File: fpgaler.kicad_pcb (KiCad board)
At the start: 4 copper layers, 100 x 100 mm, 287 parts, among them J1 USB_C_Receptacle_USB2.0, J3 JTAG, J4 FTDI_RST, J5 VGA, J6 DB9 Expander, J7 DB9 Expander, Q1 BC817, SW1 RotaryEncoder_Switch, SW2 RotaryEncoder_Switch, SW3 K1, SW4 K2, SW5 PROGRAMN, SW6 K3, SW7 FPGA GSRN, SW8 K4, U1 TLV62569DRL, U10 XC6206PxxxMR, U11 IS62WV51216BLL-55TLI, U2 TLV62569DRL, U3 NCP115-2.5, U5 93LC56BT-I/OT, U6 FT2232HL, U7 CAT24C128, U8 LFE5U-25F-8MG285C, U9 W25Q128JVP, X1 27MHz, Y1 7M-12.000MAAJ

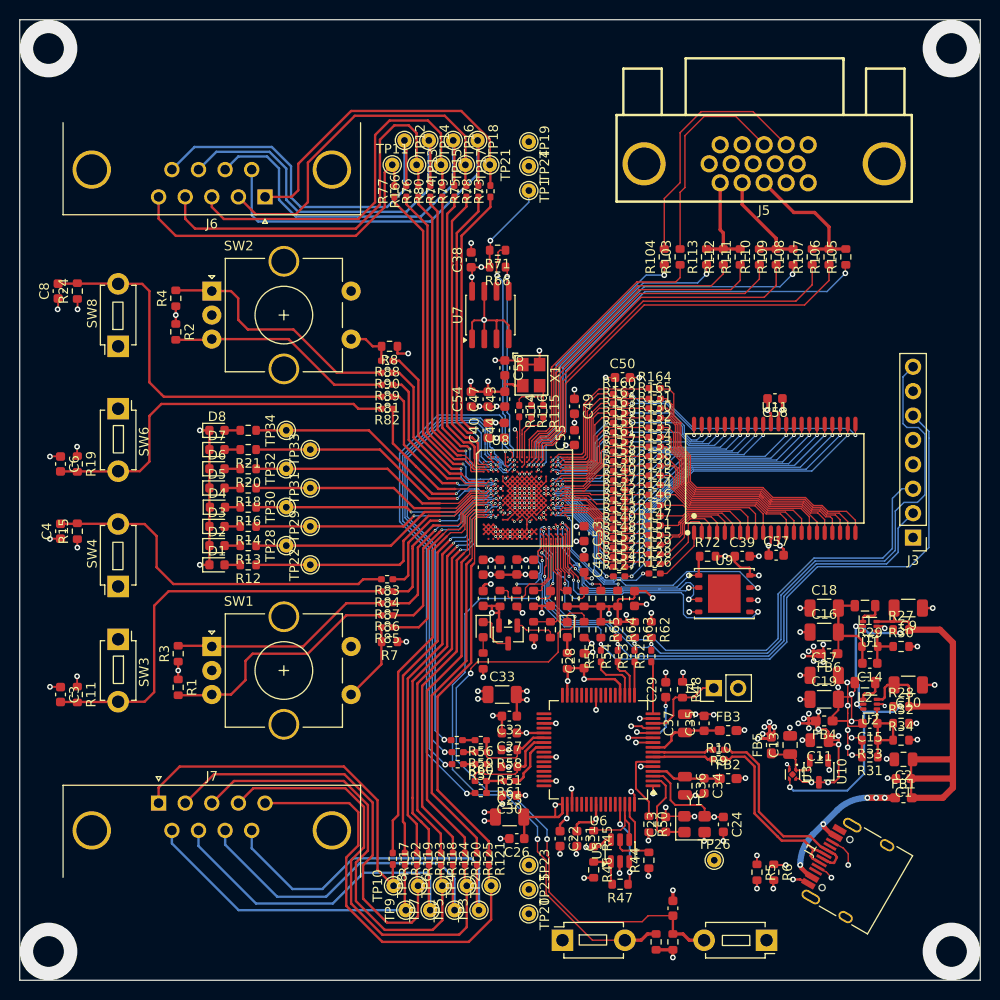
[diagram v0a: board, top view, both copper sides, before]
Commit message: Place planes
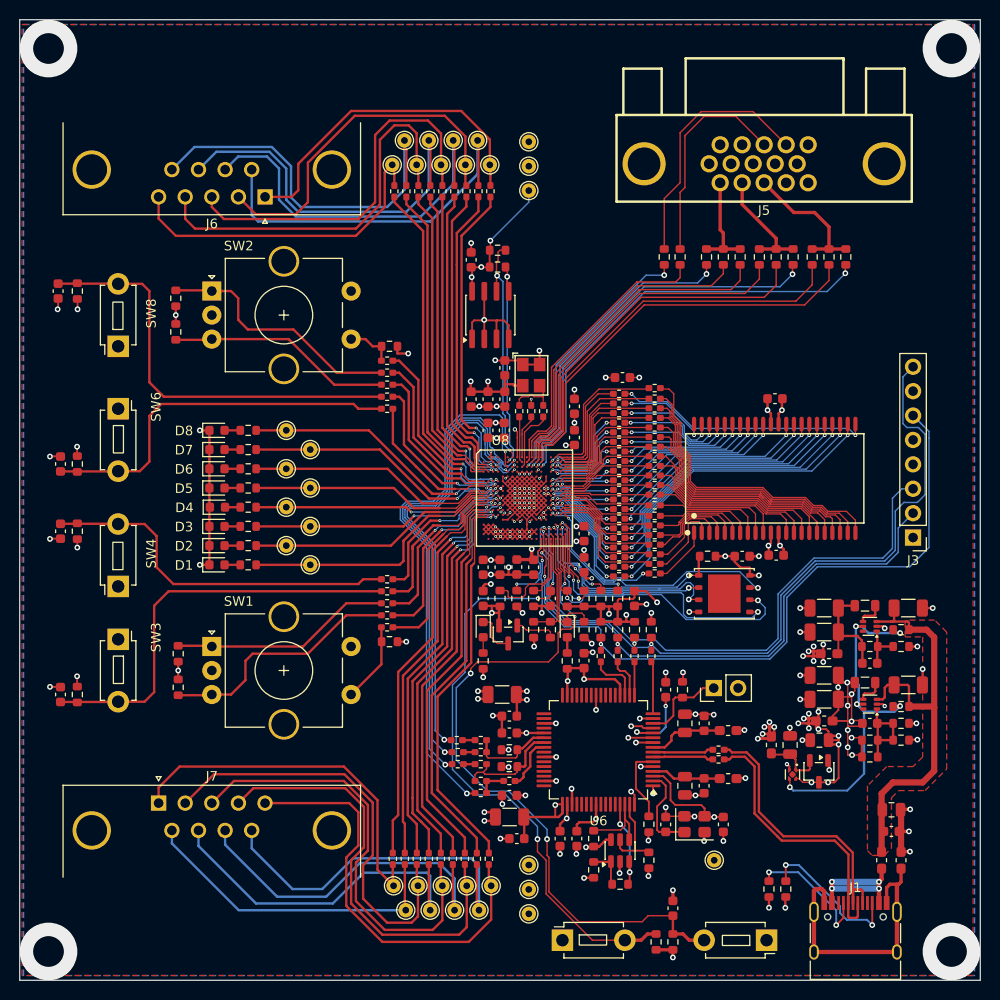
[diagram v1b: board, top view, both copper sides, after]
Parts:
- added FB7: 15Ω@100MHz, Inductor_SMD:L_0603_1608Metric_Pad1.05x0.95mm_HandSolder, F.Cu at (171.8, 132.5)
- moved FB1 6.89 mm to (169.7, 132.5), turned to 90 degrees
- moved J1 6.85 mm to (167.0, 141.0), turned to 0 degrees
- moved C1 5.64 mm to (170.8, 129.5), turned to 0 degrees
- moved C2 5.40 mm to (170.8, 127.2), turned to 0 degrees
- moved R5 3.47 mm to (159.8, 135.5)
- moved R6 1.82 mm to (158.0, 135.5)
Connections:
- J1 pad A1: GND -> Net-(J1-SHIELD)
- J1 pad A12: GND -> Net-(J1-SHIELD)
- J1 pad B1: GND -> Net-(J1-SHIELD)
- J1 pad B12: GND -> Net-(J1-SHIELD)
- J1 pad S1: GND -> Net-(J1-SHIELD)
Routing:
- net Net-(J1-SHIELD): track 0.00 -> 29.3 mm
- net SPI_CONFIG_SCK: track 7.57 -> 32.7 mm, vias 1 -> 2
- net +1.1V: track 77.3 -> 92.2 mm
- net GND: track 1061.2 -> 1075.6 mm, vias 123 -> 122
- net +5V: track 54.9 -> 44.6 mm
- net /USB_N: track 19.6 -> 29.1 mm
- net /USB_P: track 21.3 -> 29.8 mm
- net +2.5V: track 141.8 -> 149.8 mm
- net Net-(J1-CC1): track 8.64 -> 13.7 mm
- net /V_USB: track 19.2 -> 15.7 mm, vias 5 -> 4
- net Net-(J1-CC2): track 14.1 -> 16.0 mm
- net +3.3V: track 590.5 -> 592.1 mm
- net Net-(U8G-PB13B/CS1N): track 9.23 -> 9.89 mm
- added copper zone on In2.Cu, net +1.1V
- added copper zone on In1.Cu, net +2.5V
- added copper zone on In2.Cu, net +3.3V
- added copper zone on F.Cu, net +5V
- added copper zone on B.Cu, net GND
- added copper zone on F.Cu, net GND
- added copper zone on In1.Cu, net GND
